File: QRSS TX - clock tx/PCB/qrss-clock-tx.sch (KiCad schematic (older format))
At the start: 1 part

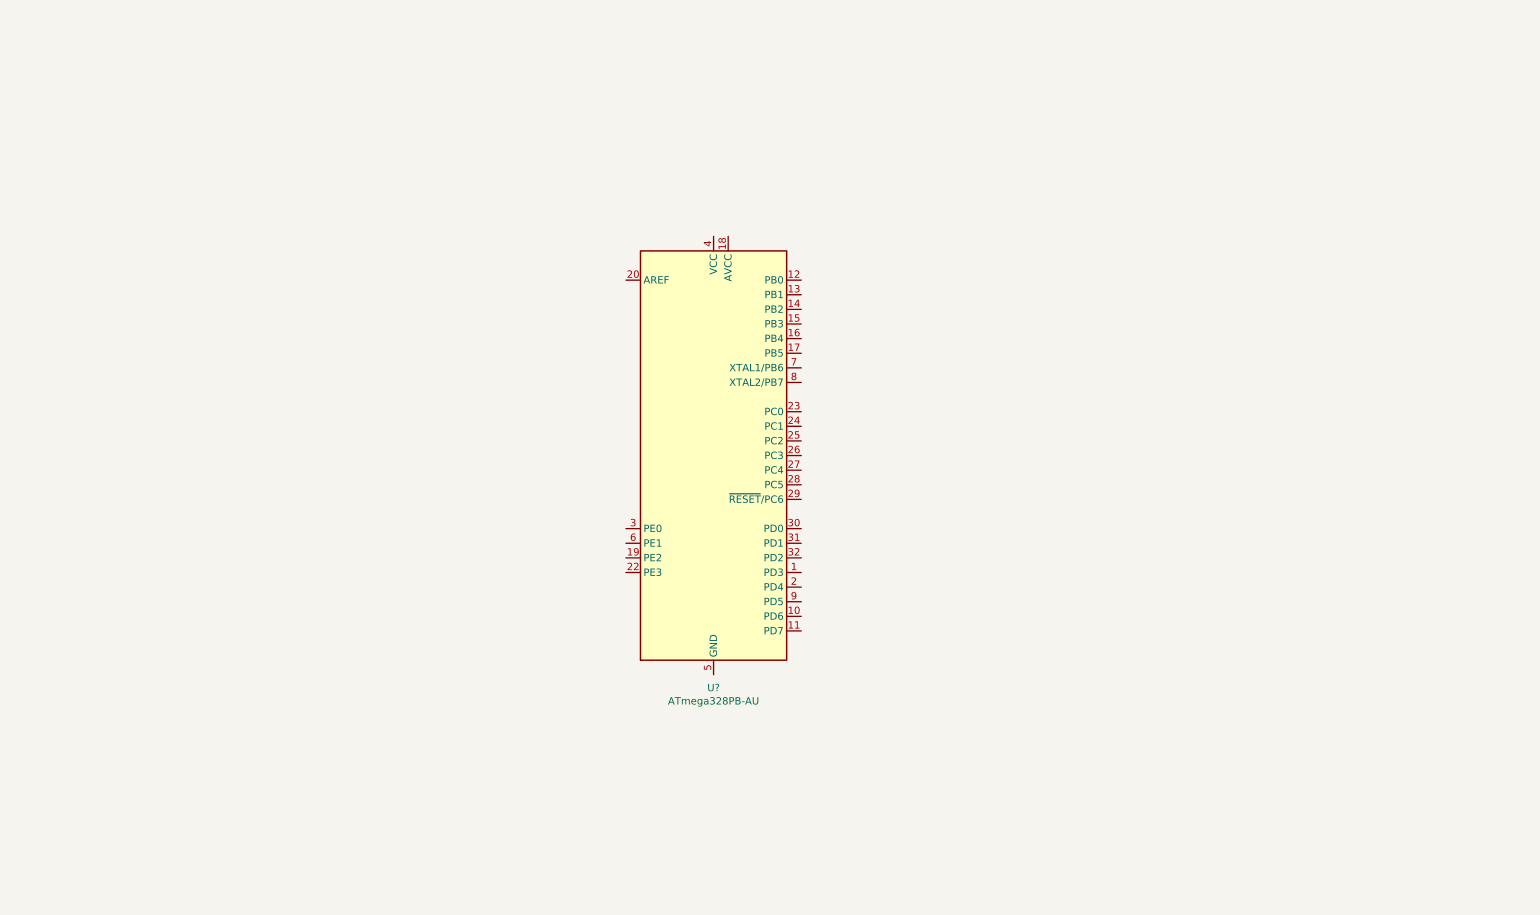
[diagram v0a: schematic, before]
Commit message: update QRSS TX schematic
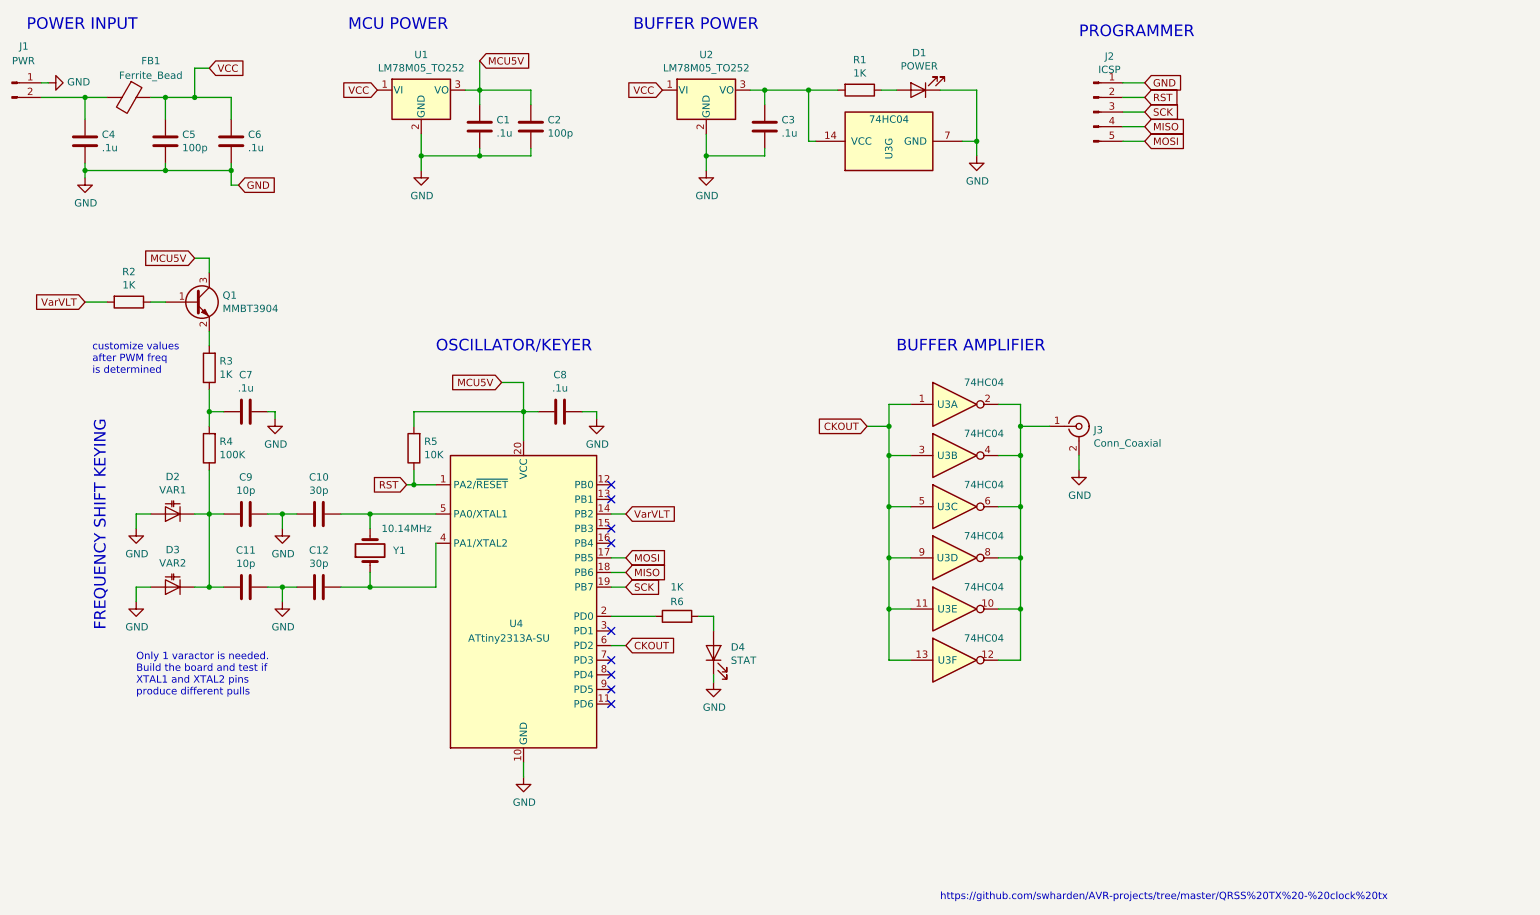
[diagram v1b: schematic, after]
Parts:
- removed U?: ATmega328PB-AU, Package_QFP:TQFP-32_7x7mm_P0.8mm, symbol MCU_Microchip_ATmega:ATmega328PB-AU
- added C1, C3, C4, C6, C7, C8: .1u, symbol Device:C
- added C10, C12: 30p, symbol Device:C
- added C11, C9: 10p, symbol Device:C
- added C2, C5: 100p, symbol Device:C
- added D1: POWER, symbol Device:LED
- added D2: VAR1, symbol Device:D_Capacitance
- added D3: VAR2, symbol Device:D_Capacitance
- added D4: STAT, symbol Device:LED
- added FB1: Ferrite_Bead, symbol Device:Ferrite_Bead
- added J1: PWR, symbol Connector:Conn_01x02_Male
- added J2: ICSP, symbol Connector:Conn_01x05_Male
- added J3: Conn_Coaxial, symbol Connector:Conn_Coaxial
- added Q1: MMBT3904, Package_TO_SOT_SMD:SOT-23, symbol Transistor_BJT:MMBT3904
- added R1, R2, R3, R6: 1K, symbol Device:R
- added R4: 100K, symbol Device:R
- added R5: 10K, symbol Device:R
- added U1, U2: LM78M05_TO252, Package_TO_SOT_SMD:TO-252-2, symbol Regulator_Linear:LM78M05_TO252
- added U3: 74HC04, symbol 74xx:74HC04
- added U4: ATtiny2313A-SU, Package_SO:SOIC-20W_7.5x12.8mm_P1.27mm, symbol MCU_Microchip_ATtiny:ATtiny2313A-SU
- added Y1: 10.14MHz, symbol Device:Crystal
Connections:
- new net: R6.1, U4.2 (PD0)
- new net: C12.1, U4.4 (PA1/XTAL2), Y1.1
- new net: C10.1, U4.5 (PA0/XTAL1), Y1.2
- new net: C11.2, C9.2, D2.1 (K), D3.1 (K), R4.1
- new net: C4.1, FB1.2, J1.2 (Pin_2)
- new net: D1.2 (A), R1.1
- new net: C3.1, R1.2, U2.3 (VO), U3.14 (VCC)
- new net: C7.2, R3.1, R4.2
- new net: Q1.1 (B), R2.1
- new net: D4.2 (A), R6.2
- new net: J3.1 (In), U3.10, U3.12, U3.2, U3.4, U3.6, U3.8
- new net: Q1.2 (E), R3.2
- new net CKOUT: U3.1, U3.11, U3.13, U3.3, U3.5, U3.9, U4.6 (PD2)
- new net GND: C1.2, C10.2, C11.1, C12.2, C2.2, C3.2, C4.2, C5.2, C6.2, C7.1, C8.2, C9.1, D1.1 (K), D2.2 (A), D3.2 (A), D4.1 (K), J1.1 (Pin_1), J2.1 (Pin_1), J3.2 (Ext), U1.2 (GND), U2.2 (GND), U3.7 (GND), U4.10 (GND)
- new net MCU5V: C1.1, C2.1, C8.1, Q1.3 (C), R5.2, U1.3 (VO), U4.20 (VCC)
- new net MISO: J2.4 (Pin_4), U4.18 (PB6)
- new net MOSI: J2.5 (Pin_5), U4.17 (PB5)
- new net RST: J2.2 (Pin_2), R5.1, U4.1 (PA2/~RESET)
- new net SCK: J2.3 (Pin_3), U4.19 (PB7)
- new net VCC: C5.1, C6.1, FB1.1, U1.1 (VI), U2.1 (VI)
- new net VarVLT: R2.2, U4.14 (PB2)
- no-connect marks 0 -> 9
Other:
- note added: "BUFFER AMPLIFIER"
- note added: "BUFFER POWER"
- note added: "FREQUENCY SHIFT KEYING"
- note added: "MCU POWER"
- note added: "OSCILLATOR/KEYER"
- note added: "Only 1 varactor is needed.\nBuild the board and test if\nXTAL1 and XTAL2 pins\nproduce different pulls"
- note added: "POWER INPUT"
- note added: "PROGRAMMER"
- note added: "customize values\nafter PWM freq\nis determined"
- note added: "https://github.com/swharden/AVR-projects/tree/master/QRSS%20TX%20-%20clock%20tx"
